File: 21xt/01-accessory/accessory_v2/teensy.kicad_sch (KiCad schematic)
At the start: 12 parts, among them Q3 NMOS, U1 DEV-16771, U2 TPS22915BYFPR

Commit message: comments for revision added
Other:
- note added: "actually is this intended for the usb connector on the teensy? because if it is, then the usb cannot back power the board and blow up your buck converter if you leave the shottky i told you to remove, but even then, the buck converter can blow up the USB line or just overvolt it because the usb does not get disconnected"
- note added: "also if we have no power on the car, but have power on usb, will this turn on? it seems to me that if the connector is plugged in then ls_en is grounded so the gate opens, but there is no power"
- note added: "also you need to add the 4 pin m8 connector for getting the usb power to the teensy, though I suppose this functions for powering the teensy via the usb connector on the teensy board"
- note added: "i dont think these are the right connections for the usb grounding"
- note added: "i dont think you have connected all of the digital pins d4,5,6"
- note added: "i think i am impartial to the case where we are connecting to the teensy via the microusb on the board but if you wanted to have a proper load switch for the m8 connector that you are exposing, then i think you would need the load switch on that line: ie if the ls_en pin is activated then turn off the m8 power,"
- note added: "it becomes a bit more complicated if you wanted to support the USB connector on the board, in that case, you probably have to have the USB power always be the source for everything when its plugged in or have to snip the trace in order to control that connection, at the very least i think you have to model the m8 connector and determine which of that connector and the big bulkhead are dominant an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"
- note added: "or hallfx3"
- note added: "shouldnt the buck converter have precedent over the usb power for example: if the usb is higher voltage than buck, then the signals will exceed the threshold for levels on the usb, if the buck converter is higher though, then the signalling on the usb side may not reach high enough. also, we want no interruption when you plug in and need to switch tho id if that is significant"
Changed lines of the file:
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@@
     (stroke (width 0) (type default))
+  )
+  (arc (start 313.69 53.34) (mid 254.2256 96.5696) (end 181.61 85.09)
+    (stroke (width 0) (type default))
+    (fill (type none))
+  )
+  (arc (start 312.42 54.61) (mid 243.3139 81.7468) (end 175.26 52.07)
+    (stroke (width 0) (type default))
+    (fill (type none))
+  )
+  (arc (start -6.35 22.86) (mid 25.5167 29.747) (end 43.18 57.15)
+    (stroke (width 0) (type default))
+    (fill (type none))
+  )
+  (arc (start 313.69 109.22) (mid 222.2951 150.7967) (end 128.27 115.57)
+    (stroke (width 0) (type default))
+    (fill (type none))
+  )
+  (arc (start 313.69 54.61) (mid 263.349 134.2339) (end 171.45 154.94)
+    (stroke (width 0) (type default))
+    (fill (type none))
   )
   (rectangle (start 27.94 35.56) (end 127 85.09)
@@
     (effects (font (size 1.27 1.27)) (justify left bottom))
   )
+  (text "it becomes a bit more complicated if you wanted to support the USB\nconnector on the board, in that case, you probably have to have\nthe USB power always be the source for everything when its plugged\nin or have to snip the trace in order to control that connection,\nat the very least i think you have to model the m8 connector\nand determine which of that connector and the big bulkhead are dominant\nand possible just ignore the usb, but maximally, this would require two\nload switches and possibly snipping the connection, but i think we can\nget around that by just asuming the usb connector is only for off board\ncases and the primary modality of programming this guy is through the\nm8 connector"
+    (at -74.93 127 0)
+    (effects (font (size 1.27 1.27)) (justify left bottom))
+  )
   (text "Nominal: 0\nHigh: 5 V" (at 30.48 76.2 0)
+    (effects (font (size 1.27 1.27)) (justify left bottom))
+  )
+  (text "shouldnt the buck converter have precedent over the usb power\nfor example: if the usb is higher voltage than buck, then\nthe signals will exceed the threshold for levels on the usb,\nif the buck converter is higher though, then the signalling \non the usb side may not reach high enough. also, we want no\ninterruption when you plug in and need to switch tho id if \nthat is significant"
+    (at -71.12 21.59 0)
+    (effects (font (size 1.27 1.27)) (justify left bottom))
+  )
+  (text "actually is this intended for the usb connector\non the teensy? because if it is, then the usb\ncannot back power the board and blow up your \nbuck converter if you leave the shottky i told\nyou to remove, but even then, the buck converter\ncan blow up the USB line or just overvolt it\nbecause the usb does not get disconnected"
+    (at -80.01 72.39 0)
     (effects (font (size 1.27 1.27)) (justify left bottom))
   )
@@
     (effects (font (size 1.27 1.27)) (justify left bottom))
   )
+  (text "or hallfx3" (at 313.69 114.3 0)
+    (effects (font (size 1.27 1.27)) (justify left bottom))
+  )
+  (text "i dont think you have connected all of the digital pins d4,5,6"
+    (at 313.69 110.49 0)
+    (effects (font (size 1.27 1.27)) (justify left bottom))
+  )
+  (text "also you need to add the 4 pin m8 connector\nfor getting the usb power to the teensy,\nthough I suppose this functions for powering the teensy\nvia the usb connector on the teensy board"
+    (at -69.85 50.8 0)
+    (effects (font (size 1.27 1.27)) (justify left bottom))
+  )
+  (text "i think i am impartial to the case where we are connecting\nto the teensy via the microusb on the board but\nif you wanted to have a proper load switch for the\nm8 connector that you are exposing, then i think you would need\nthe load switch on that line: ie if the ls_en pin is activated\nthen turn off the m8 power,\n"
+    (at -78.74 97.79 0)
+    (effects (font (size 1.27 1.27)) (justify left bottom))
+  )
+  (text "i dont think these are the right connections for the usb grounding"
+    (at 317.5 54.61 0)
+    (effects (font (size 1.27 1.27)) (justify left bottom))
+  )
+  (text "also if we have no power on the car, but have power on usb, will this turn on?\nit seems to me that if the connector is plugged in then\nls_en is grounded so the gate opens, but there is no power "
+    (at -76.2 34.29 0)
+    (effects (font (size 1.27 1.27)) (justify left bottom))
+  )

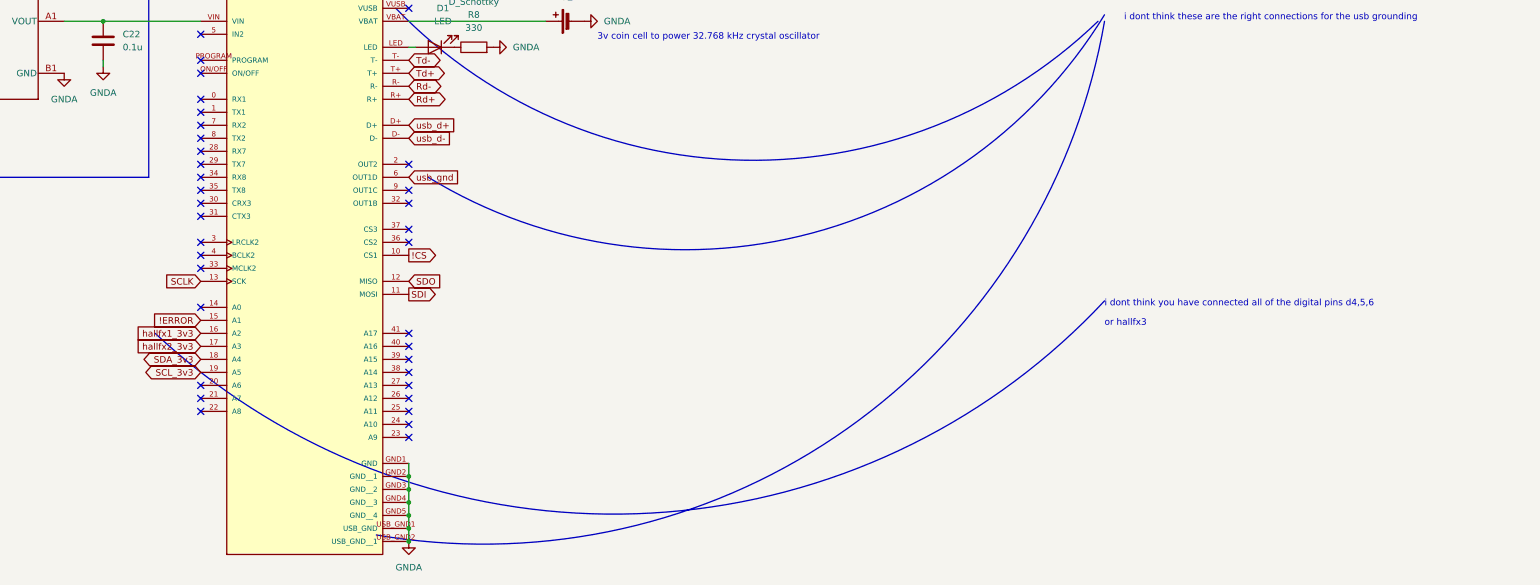
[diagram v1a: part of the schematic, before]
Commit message: Addressed some comments
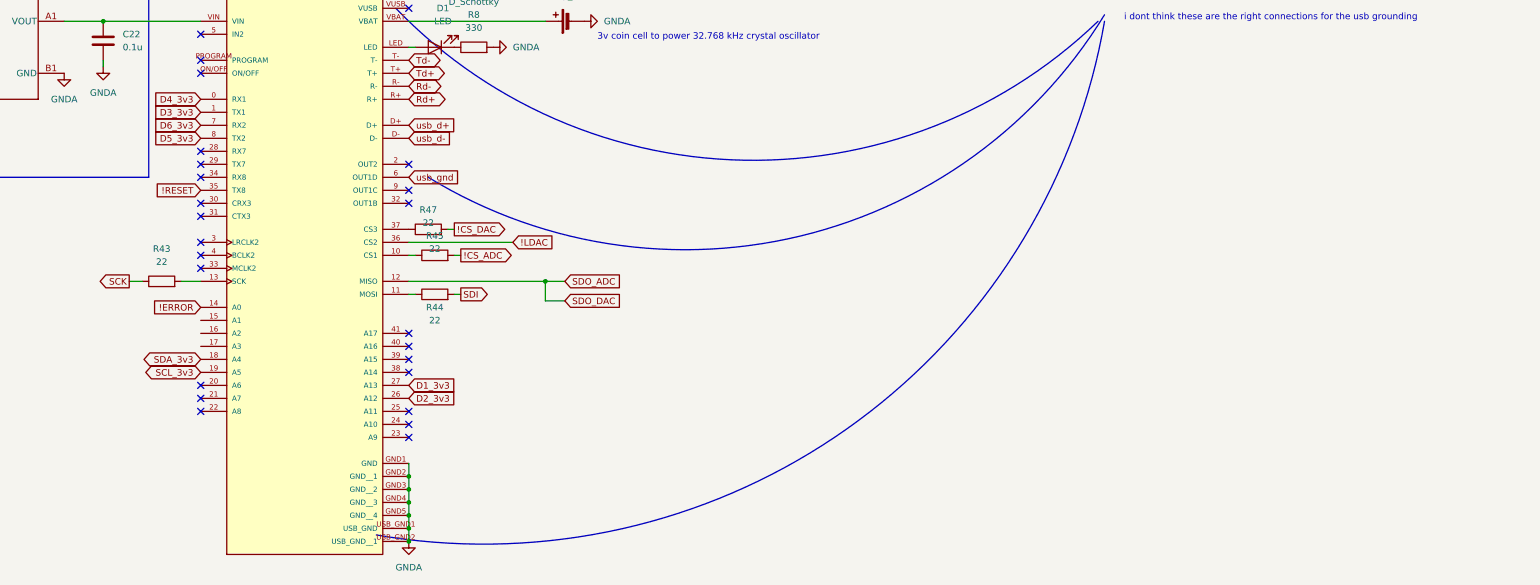
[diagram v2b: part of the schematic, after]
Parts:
- added R43, R44, R45, R47: 22, symbol Device:R
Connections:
- net !ERROR: now also U1.14 (A0); no longer U1.15 (A1)
- net SDI: now also R44.2; no longer U1.11 (MOSI)
- net D4_3v3: now reaches U1.0 (RX1)
- net D3_3v3: now reaches U1.1 (TX1)
- net D2_3v3: now reaches U1.26 (A12)
- net D1_3v3: now reaches U1.27 (A13)
- net !RESET: now reaches U1.35 (TX8)
- net !LDAC: now reaches U1.36 (CS2)
- net at U1.37 (CS3): now also R47.1
- net D6_3v3: now reaches U1.7 (RX2)
- net D5_3v3: now reaches U1.8 (TX2)
- net !CS: no longer names the net of U1.10 (CS1)
- net !CS: now also R45.1
- net SCLK: no longer names the net of U1.13 (SCK)
- net SCLK: now also R43.2
- net SDO renamed SDO_ADC
- net hallfx1_3v3: no longer names the net of U1.16 (A2)
- net hallfx2_3v3: no longer names the net of U1.17 (A3)
- new net: R44.1, U1.11 (MOSI)
- new net !CS_ADC: R45.2
- new net !CS_DAC: R47.2
- new net SCK: R43.1
- no-connect marks 38 -> 28
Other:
- note removed: "i dont think you have connected all of the digital pins d4,5,6"
- note removed: "or hallfx3"

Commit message: added files
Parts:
- removed D4: D_Schottky, Diode_SMD:D_0603_1608Metric, symbol Device:D_Schottky
- removed Q3: NMOS, symbol Simulation_SPICE:NMOS
- added Q3: BSS138, Package_TO_SOT_SMD:SOT-23, symbol Transistor_FET:BSS138
- C22, C44: footprint Capacitor_SMD:C_0603_1608Metric -> Capacitor_SMD:C_0402_1005Metric
- R19, R20, R43, R44, R45, R47: footprint (none) -> Resistor_SMD:R_0603_1608Metric
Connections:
- net 3v3: now also U1.3.3V_2 (3.3V__1)
- net GNDA: now also Q3.2 (S)
- net LS_EN: now also Q3.1 (G)
- net at R19.2, U2.B2 (ON): now also Q3.3 (D)
- net at U1.23 (A9): now also D1.2 (A)
- net GPIO/INT1_3v3: now reaches U1.24 (A10)
- net GPIO/INT2_3v3: now reaches U1.25 (A11)
- net at U1.LED: no longer D1.2 (A)
- net 5v_usb: now reaches U1.VUSB
- net usb_d+: no longer names the net of U1.D+
- net usb_d-: no longer names the net of U1.D-
- net usb_gnd: no longer names the net of U1.6 (OUT1D)
- no-connect marks 28 -> 31
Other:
- note added: "LS_EN = 0 -> Buck converter is connected LS_EN = 5 -> Buck converter is not connected"
- note removed: "Nominal: 0 High: 5 V"
- note removed: "actually is this intended for the usb connector on the teensy? because if it is, then the usb cannot back power the board and blow up your buck converter if you leave the shottky i told you to remove, but even then, the buck converter can blow up the USB line or just overvolt it because the usb does not get disconnected"
- note removed: "also if we have no power on the car, but have power on usb, will this turn on? it seems to me that if the connector is plugged in then ls_en is grounded so the gate opens, but there is no power"
- note removed: "also you need to add the 4 pin m8 connector for getting the usb power to the teensy, though I suppose this functions for powering the teensy via the usb connector on the teensy board"
- note removed: "i dont think these are the right connections for the usb grounding"
- note removed: "i think i am impartial to the case where we are connecting to the teensy via the microusb on the board but if you wanted to have a proper load switch for the m8 connector that you are exposing, then i think you would need the load switch on that line: ie if the ls_en pin is activated then turn off the m8 power,"
- note removed: "it becomes a bit more complicated if you wanted to support the USB connector on the board, in that case, you probably have to have the USB power always be the source for everything when its plugged in or have to snip the trace in order to control that connection, at the very least i think you have to model the m8 connector and determine which of that connector and the big bulkhead are dominant an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"
- note removed: "shouldnt the buck converter have precedent over the usb power for example: if the usb is higher voltage than buck, then the signals will exceed the threshold for levels on the usb, if the buck converter is higher though, then the signalling on the usb side may not reach high enough. also, we want no interruption when you plug in and need to switch tho id if that is significant"

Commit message: some work, a bit scuffed
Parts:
- removed Q3: BSS138, Package_TO_SOT_SMD:SOT-23, symbol Transistor_FET:BSS138
- added Q3: NMOS, Package_TO_SOT_SMD:SOT-23-3, symbol Simulation_SPICE:NMOS
- added R41, R42, R46, R48, R49: 20R, Resistor_SMD:R_0402_1005Metric, symbol Device:R
- BT1: footprint Battery:BatteryHolder_Keystone_1060_1x2032 -> 21xt_footprints:1220 holder
- R19, R20, R8: footprint Resistor_SMD:R_0603_1608Metric -> Resistor_SMD:R_0402_1005Metric
- R43, R44, R45, R47: value 22 -> 20R; footprint Resistor_SMD:R_0603_1608Metric -> Resistor_SMD:R_0402_1005Metric
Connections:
- net !ERROR: now also U1.30 (CRX3); no longer U1.14 (A0)
- net !LDAC: now also R48.1; no longer U1.36 (CS2)
- net 3v3: now also U1.3.3V_3 (3.3V__2)
- net D1_3v3: now also R46.1
- net D2_3v3: now also R47.1
- net D3_3v3: now also R44.1, U1.39 (A15); no longer U1.1 (TX1)
- net D4_3v3: now also R45.1, U1.38 (A14); no longer U1.0 (RX1)
- net D5_3v3: now also U1.41 (A17); no longer U1.8 (TX2)
- net D6_3v3: now also U1.40 (A16); no longer U1.7 (RX2)
- net GNDA: no longer BT1.2 (-), C22.1, C44.1, R20.2, U1.GND1 (GND), U1.GND2 (GND__1), U1.GND3 (GND__2), U1.GND4 (GND__3), U1.GND5 (GND__4), U1.USB_GND1 (USB_GND), U1.USB_GND2 (USB_GND__1), U2.B1 (GND)
- net GPIO/INT1_3v3: now also U1.0 (RX1); no longer U1.24 (A10)
- net GPIO/INT2_3v3: now also U1.1 (TX1); no longer U1.25 (A11)
- net LS_EN: now also Q3.2 (G)
- net at U1.37 (CS3): no longer R47.1
- net at U1.23 (A9): no longer D1.2 (A)
- net at U1.10 (CS1): now also R49.1; no longer R45.1
- net at R19.2, U2.B2 (ON): now also Q3.1 (D)
- net at U1.11 (MOSI): now also R42.1; no longer R44.1
- net SYNC: now reaches U1.31 (CTX3)
- net at U1.32 (OUT1B): now also R48.2
- net usb_d+: now reaches U1.D+
- net usb_d-: now reaches U1.D-
- net at U1.LED: now also D1.2 (A)
- net !CS_ADC renamed CS-DAC
- net !CS_DAC renamed MOSI1
- net !RESET: no longer names the net of U1.35 (TX8)
- net 5v_usb: no longer names the net of U1.VUSB
- net SCK renamed SCLK
- net SDI renamed MISO1
- net SDO_ADC: no longer names the net of U1.12 (MISO)
- net SDO_ADC: now also R41.1
- new net !CS: R49.2
- new net GNDD: BT1.2 (-), C22.1, C44.1, Q3.3 (S), R20.2, U1.GND1 (GND), U1.GND2 (GND__1), U1.GND3 (GND__2), U1.GND4 (GND__3), U1.GND5 (GND__4), U2.B1 (GND)
- new net MISO: R41.2
- new net MOSI: R42.2
- new net SCLK1: R46.2
- new net usb_gnd: U1.USB_GND1 (USB_GND), U1.USB_GND2 (USB_GND__1)
- no-connect marks 31 -> 30
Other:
- note added: "Nominal: 0 High: 5 V"
- note added: "actually is this intended for the usb connector on the teensy? because if it is, then the usb cannot back power the board and blow up your buck converter if you leave the shottky i told you to remove, but even then, the buck converter can blow up the USB line or just overvolt it because the usb does not get disconnected"
- note added: "also if we have no power on the car, but have power on usb, will this turn on? it seems to me that if the connector is plugged in then ls_en is grounded so the gate opens, but there is no power"
- note added: "also you need to add the 4 pin m8 connector for getting the usb power to the teensy, though I suppose this functions for powering the teensy via the usb connector on the teensy board"
- note added: "i dont think these are the right connections for the usb grounding"
- note added: "i think i am impartial to the case where we are connecting to the teensy via the microusb on the board but if you wanted to have a proper load switch for the m8 connector that you are exposing, then i think you would need the load switch on that line: ie if the ls_en pin is activated then turn off the m8 power,"
- note added: "it becomes a bit more complicated if you wanted to support the USB connector on the board, in that case, you probably have to have the USB power always be the source for everything when its plugged in or have to snip the trace in order to control that connection, at the very least i think you have to model the m8 connector and determine which of that connector and the big bulkhead are dominant an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"
- note added: "shouldnt the buck converter have precedent over the usb power for example: if the usb is higher voltage than buck, then the signals will exceed the threshold for levels on the usb, if the buck converter is higher though, then the signalling on the usb side may not reach high enough. also, we want no interruption when you plug in and need to switch tho id if that is significant"
- note removed: "LS_EN = 0 -> Buck converter is connected LS_EN = 5 -> Buck converter is not connected"
- moved on the sheet: C22, C44, R19, R20, U2
